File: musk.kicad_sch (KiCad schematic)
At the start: 53 parts, among them J1 debug-port, J10 Conn_01x06_Male, J3 Conn_01x06_Male, J4 Conn_01x06_Male, J5 Conn_01x06_Male, J6 Conn_01x06_Male, J7 Conn_01x06_Male, J8 Conn_01x06_Male, J9 Conn_01x06_Male, K1 diode-choc, K10 diode-choc, K11 diode-choc, K12 diode-choc, K13 diode-choc, K14 diode-choc, K15 diode-choc, K16 diode-choc, K17 diode-choc, K2 diode-choc, K3 diode-choc, K4 diode-choc, K5 diode-choc, K6 diode-choc, K7 diode-choc, K8 diode-choc, K9 diode-choc, SW1 SW_Push, SW2 RotaryEncoder, U1 W25Q128, U2 ms88sf3-nrf52840, U3 LSM6DS3, U8 PMW3610

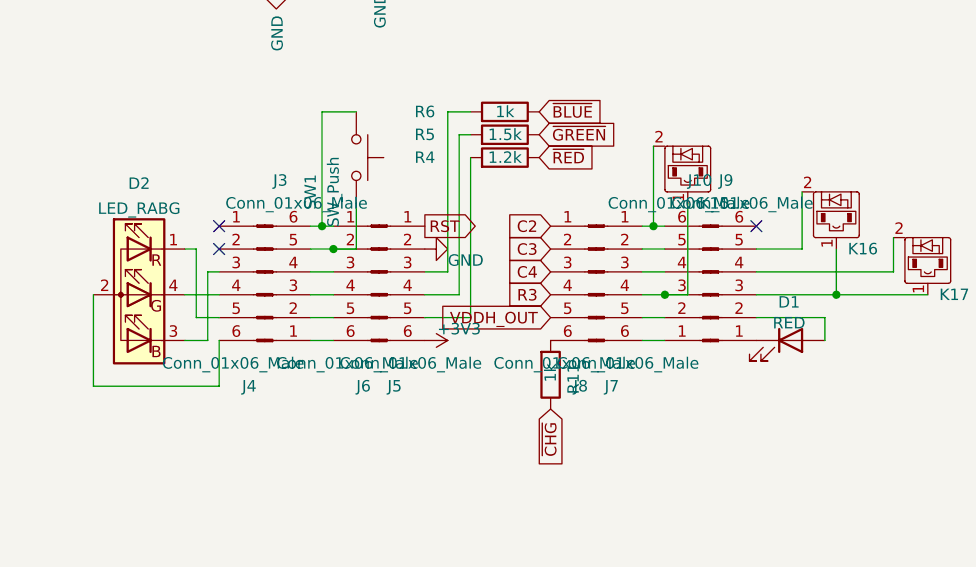
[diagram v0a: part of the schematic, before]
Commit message: top
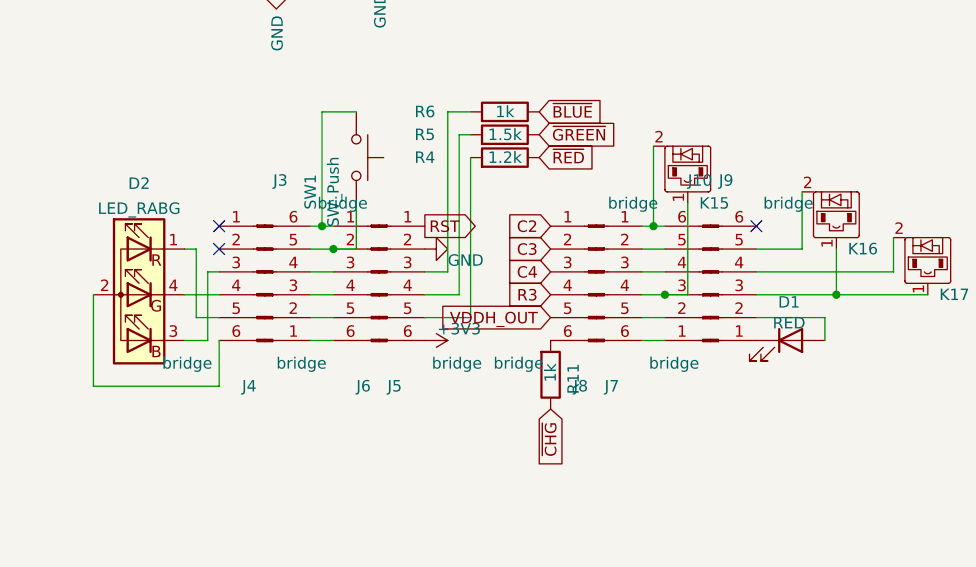
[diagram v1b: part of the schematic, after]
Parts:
- J10, J3, J4, J5, J6, J7, J8, J9: value Conn_01x06_Male -> bridge
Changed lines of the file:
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@@
       (effects (font (size 1.27 1.27)) (justify right))
     )
-    (property "Value" "Conn_01x06_Male" (id 1) (at 238.76 125.73 0)
+    (property "Value" "bridge" (id 1) (at 238.76 125.73 0)
       (effects (font (size 1.27 1.27)) (justify right))
     )
@@
       (effects (font (size 1.27 1.27)) (justify right))
     )
-    (property "Value" "Conn_01x06_Male" (id 1) (at 226.06 107.95 0)
+    (property "Value" "bridge" (id 1) (at 226.06 107.95 0)
       (effects (font (size 1.27 1.27)) (justify right))
     )
@@
       (effects (font (size 1.27 1.27)) (justify right))
     )
-    (property "Value" "Conn_01x06_Male" (id 1) (at 203.2 125.73 0)
+    (property "Value" "bridge" (id 1) (at 203.2 125.73 0)
       (effects (font (size 1.27 1.27)) (justify right))
     )
@@
       (effects (font (size 1.27 1.27)) (justify right))
     )
-    (property "Value" "Conn_01x06_Male" (id 1) (at 275.59 107.95 0)
+    (property "Value" "bridge" (id 1) (at 275.59 107.95 0)
       (effects (font (size 1.27 1.27)) (justify right))
     )
@@
       (effects (font (size 1.27 1.27)) (justify right))
     )
-    (property "Value" "Conn_01x06_Male" (id 1) (at 215.9 125.73 0)
+    (property "Value" "bridge" (id 1) (at 215.9 125.73 0)
       (effects (font (size 1.27 1.27)) (justify right))
     )
@@
       (effects (font (size 1.27 1.27)) (justify right))
     )
-    (property "Value" "Conn_01x06_Male" (id 1) (at 252.73 107.95 0)
+    (property "Value" "bridge" (id 1) (at 252.73 107.95 0)
       (effects (font (size 1.27 1.27)) (justify right))
     )
@@
       (effects (font (size 1.27 1.27)) (justify right))
     )
-    (property "Value" "Conn_01x06_Male" (id 1) (at 262.89 125.73 0)
+    (property "Value" "bridge" (id 1) (at 262.89 125.73 0)
       (effects (font (size 1.27 1.27)) (justify right))
     )
@@
       (effects (font (size 1.27 1.27)) (justify right))
     )
-    (property "Value" "Conn_01x06_Male" (id 1) (at 240.03 125.73 0)
+    (property "Value" "bridge" (id 1) (at 240.03 125.73 0)
       (effects (font (size 1.27 1.27)) (justify right))
     )
@@
     )
     (path "/13ba9cc6-feab-41e2-9f0a-09c409038987"
-      (reference "J3") (unit 1) (value "Conn_01x06_Male") (footprint "musk:bridge")
+      (reference "J3") (unit 1) (value "bridge") (footprint "musk:bridge")
     )
     (path "/25c29169-6ec4-4a25-979d-f596fdc044b9"
-      (reference "J4") (unit 1) (value "Conn_01x06_Male") (footprint "musk:bridge")
+      (reference "J4") (unit 1) (value "bridge") (footprint "musk:bridge")
     )
     (path "/12471d44-d3bf-4128-b847-f56e537242a3"
-      (reference "J5") (unit 1) (value "Conn_01x06_Male") (footprint "musk:bridge")
+      (reference "J5") (unit 1) (value "bridge") (footprint "musk:bridge")
     )
     (path "/b2e6f337-4797-4755-922d-10208728ffa5"
-      (reference "J6") (unit 1) (value "Conn_01x06_Male") (footprint "musk:bridge")
+      (reference "J6") (unit 1) (value "bridge") (footprint "musk:bridge")
     )
     (path "/cf5489a3-2bc4-4cd6-82dd-5ed37be5af94"
-      (reference "J7") (unit 1) (value "Conn_01x06_Male") (footprint "musk:bridge")
+      (reference "J7") (unit 1) (value "bridge") (footprint "musk:bridge")
     )
     (path "/fb87447a-5a57-41b1-b7c4-4666568e2348"
-      (reference "J8") (unit 1) (value "Conn_01x06_Male") (footprint "musk:bridge")
+      (reference "J8") (unit 1) (value "bridge") (footprint "musk:bridge")
     )
     (path "/84f91bd3-e4aa-4fcd-b902-b31e694e11f1"
-      (reference "J9") (unit 1) (value "Conn_01x06_Male") (footprint "musk:bridge")
+      (reference "J9") (unit 1) (value "bridge") (footprint "musk:bridge")
     )
     (path "/bde858d9-fa44-47e3-aa4a-29083efd5e88"
-      (reference "J10") (unit 1) (value "Conn_01x06_Male") (footprint "musk:bridge")
+      (reference "J10") (unit 1) (value "bridge") (footprint "musk:bridge")
     )
     (path "/06e79cfb-e062-456a-915a-aac3339d9f3e"
